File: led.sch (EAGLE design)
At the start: 46 parts, among them U1 TPS92513, U2 TPS92513

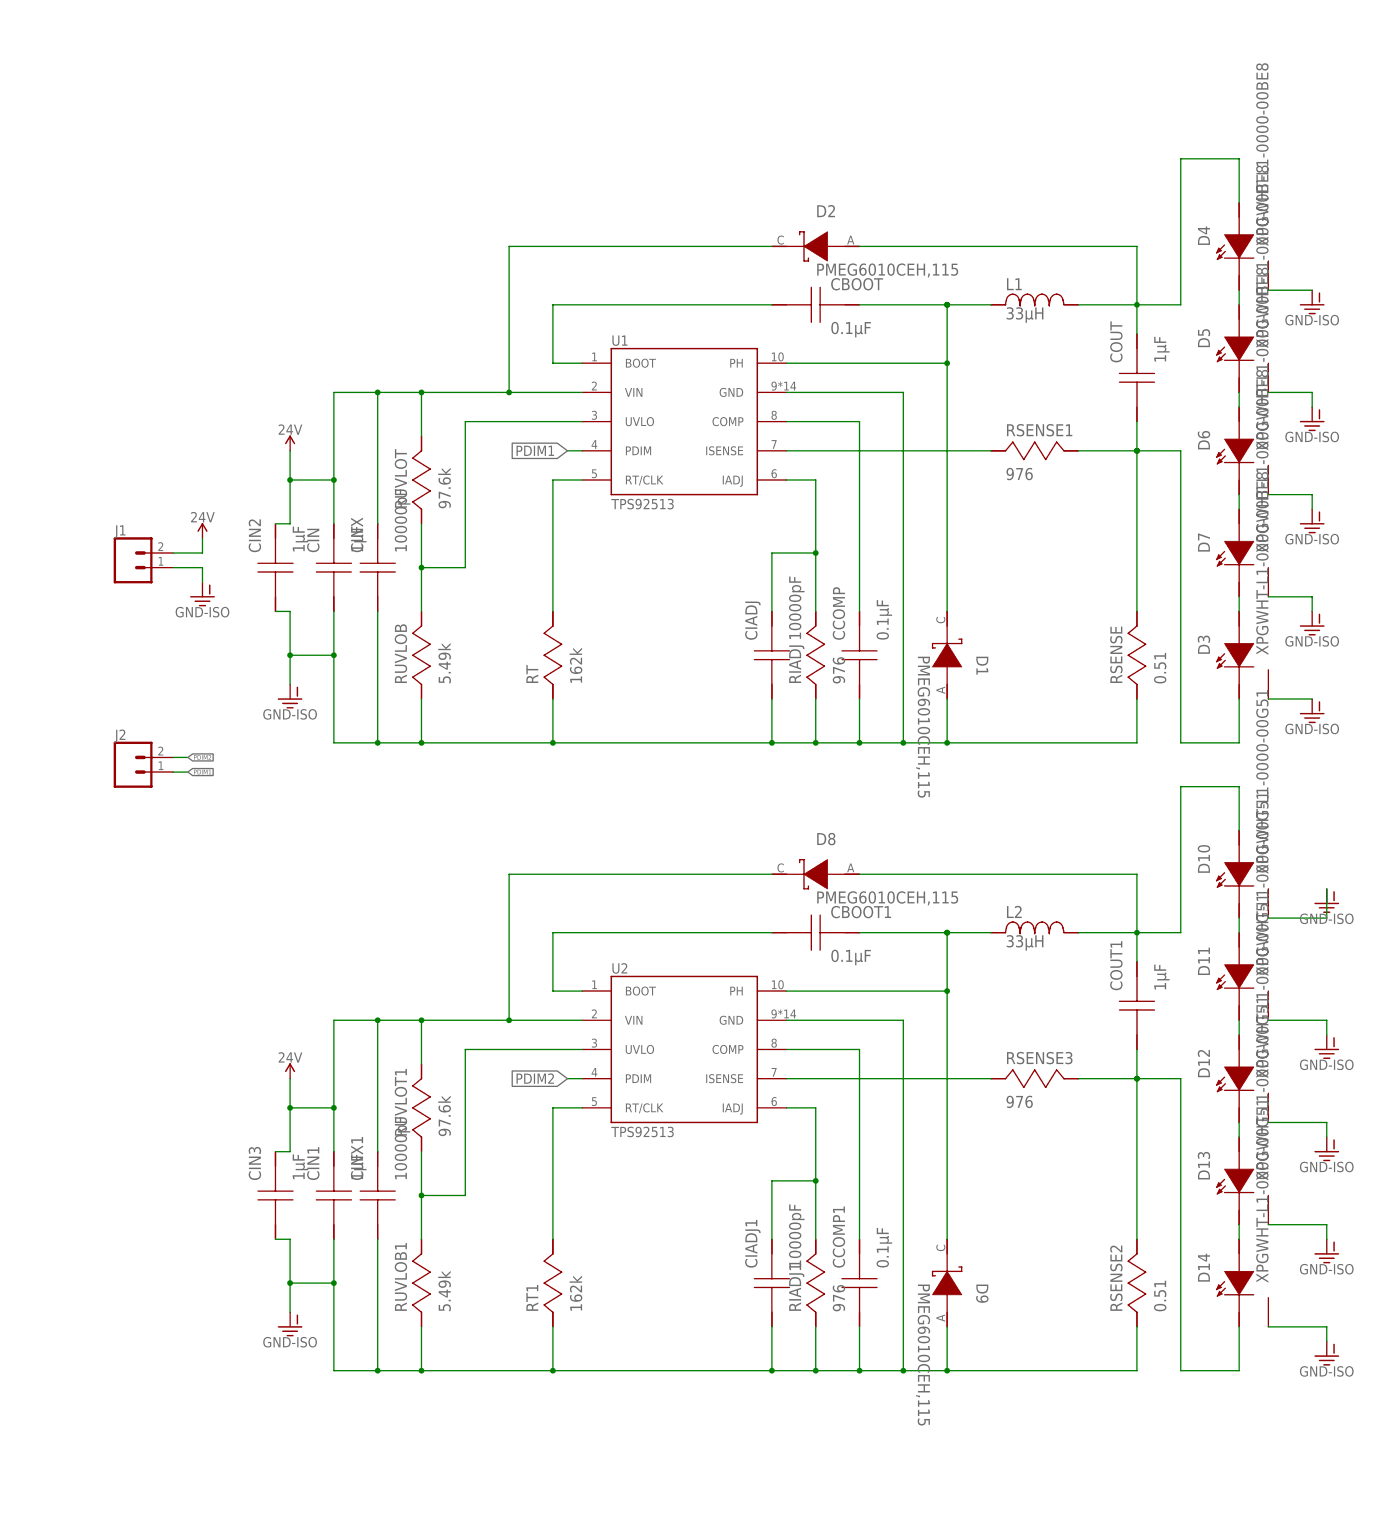
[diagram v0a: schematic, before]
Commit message: save
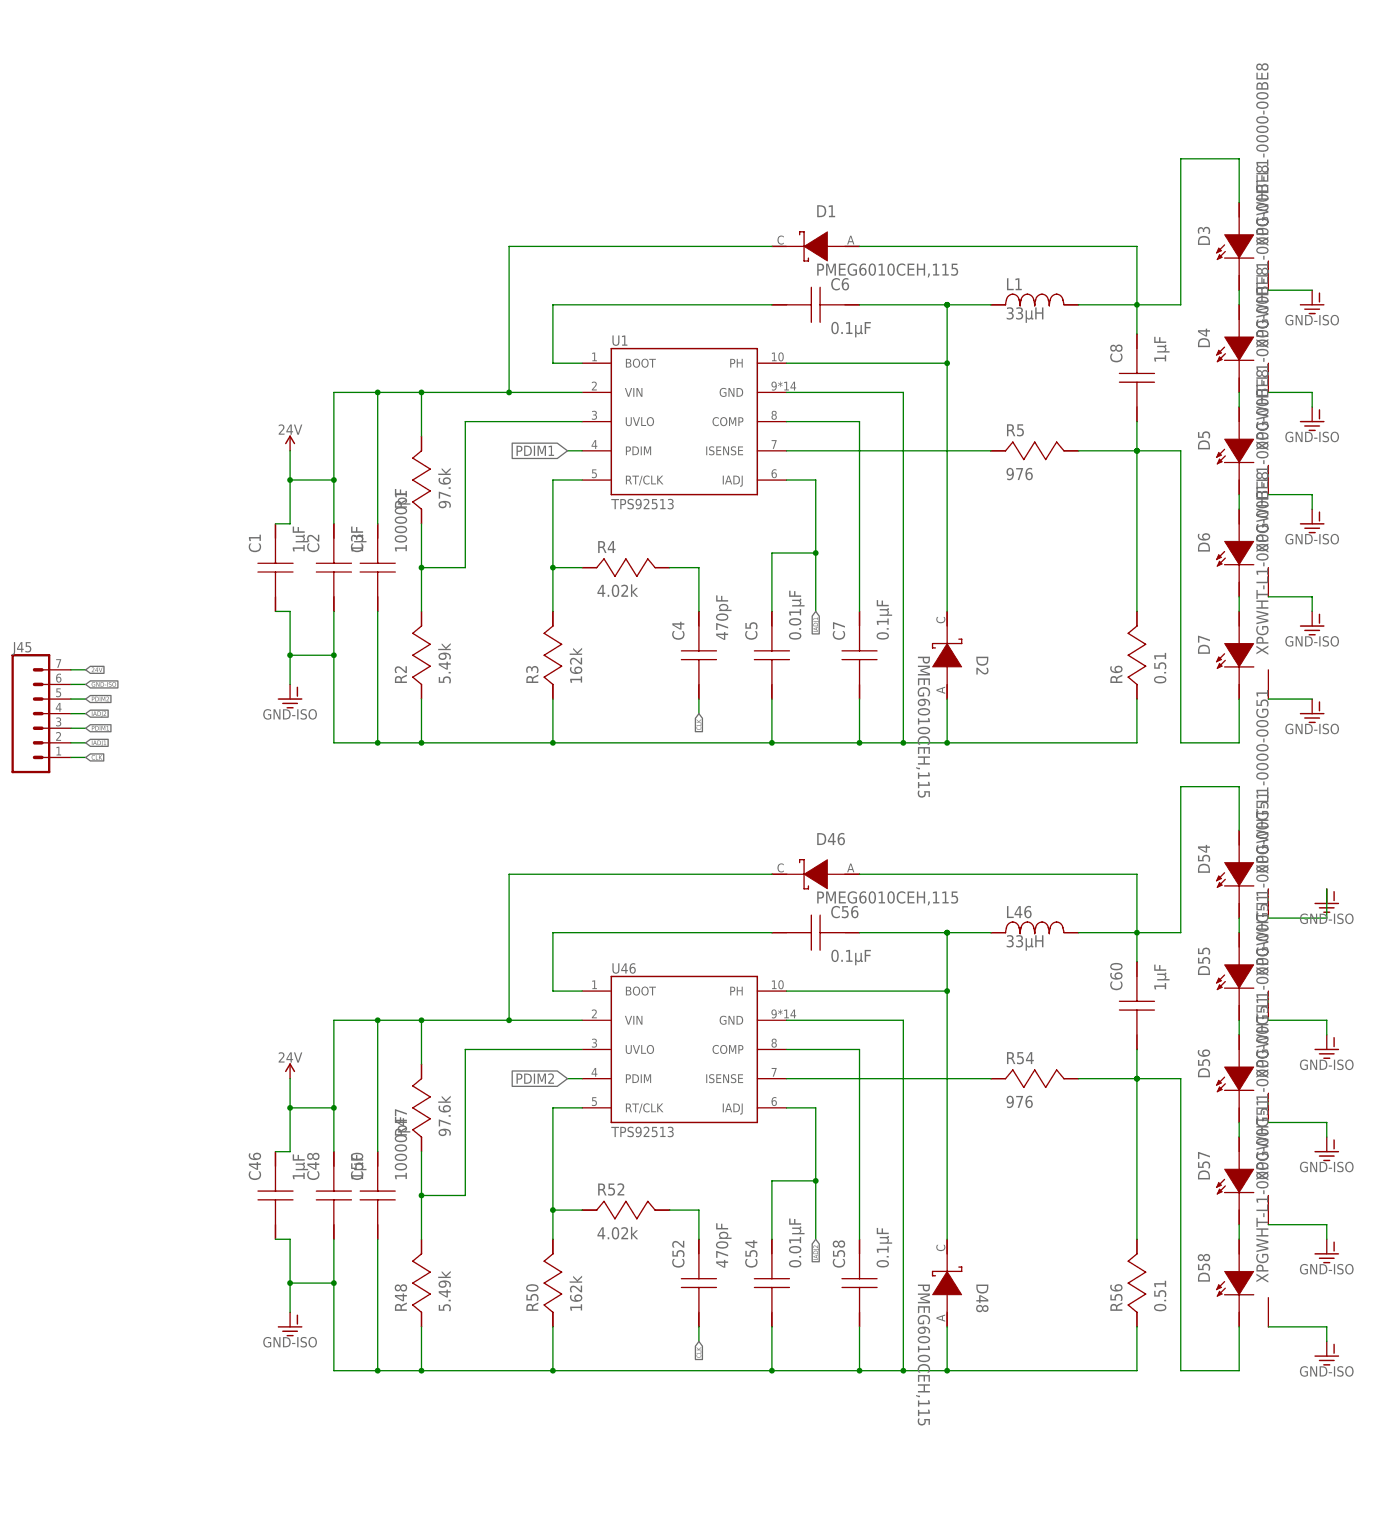
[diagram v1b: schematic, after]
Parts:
- removed CBOOT, CBOOT1: 0.1µF, derek:08053C104KAT2A
- removed J1, J2: (no value), derek:CONN_02
- removed RIADJ, RIADJ1: 976, derek:CRCW0402976RFKED
- added C4, C52: 470pF, derek:C0603X471K5RACTU
- added C56, C6: 0.1µF, derek:GRM188R71E104KA01D
- added J45: (no value), derek:CONN_07NO_SILK
- added R4, R52: 4.02k, derek:CRCW06034K02FKEA
- C5, C54: value 10000pF -> 0.01μF
- renumbered CCOMP to C7, CCOMP1 to C58, CIADJ to C5, CIADJ1 to C54, CIN to C2, CIN1 to C48, CIN2 to C1, CIN3 to C46, CINX to C3, CINX1 to C50, COUT to C8, COUT1 to C60, D10 to D54, D11 to D55, D12 to D56, D13 to D57, D14 to D58, D8 to D46, D9 to D48, L2 to L46, RSENSE to R6, RSENSE1 to R5, RSENSE2 to R56, RSENSE3 to R54, RT to R3, RT1 to R50, RUVLOB to R2, RUVLOB1 to R48, RUVLOT to R1, RUVLOT1 to R47, U2 to U46
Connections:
- removed net N$12 (its old number): D3.A, D7.C
- removed net N$2: C5.1, RIADJ.1, U1.IADJ
- removed net N$4: C54.1, RIADJ1.1, U46.IADJ
- new net CLK: C4.2, C52.2, J45.1
- new net IADJ1: C5.1, J45.2, U1.IADJ
- new net IADJ2: C54.1, J45.4, U46.IADJ
- new net N$13: D3.C, D4.A
- new net N$34: C4.1, R4.1
- new net N$36: C52.1, R52.1
- net 24V: now also D1.C, J45.7; no longer D2.C, J1.2
- net GND-ISO: now also D2.A, J45.6; no longer D1.A, J1.1, RIADJ.2, RIADJ1.2
- net N$10: now also C6.2; no longer CBOOT.2
- net N$16: now also C56.1; no longer CBOOT1.1
- net N$19: now also R52.2
- net N$21: now also C56.2; no longer CBOOT1.2
- net N$5: now also C6.1, D2.C; no longer CBOOT.1, D1.C
- net N$6: now also D7.C; no longer D3.C
- net N$7: now also D1.A, D3.A; no longer D2.A, D4.A
- net N$8: now also R4.2
- net PDIM1: now also J45.3; no longer J2.1
- net PDIM2: now also J45.5; no longer J2.2
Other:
- moved on the sheet: D1, D2, D3, D4, D5, D6, D7

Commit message: save
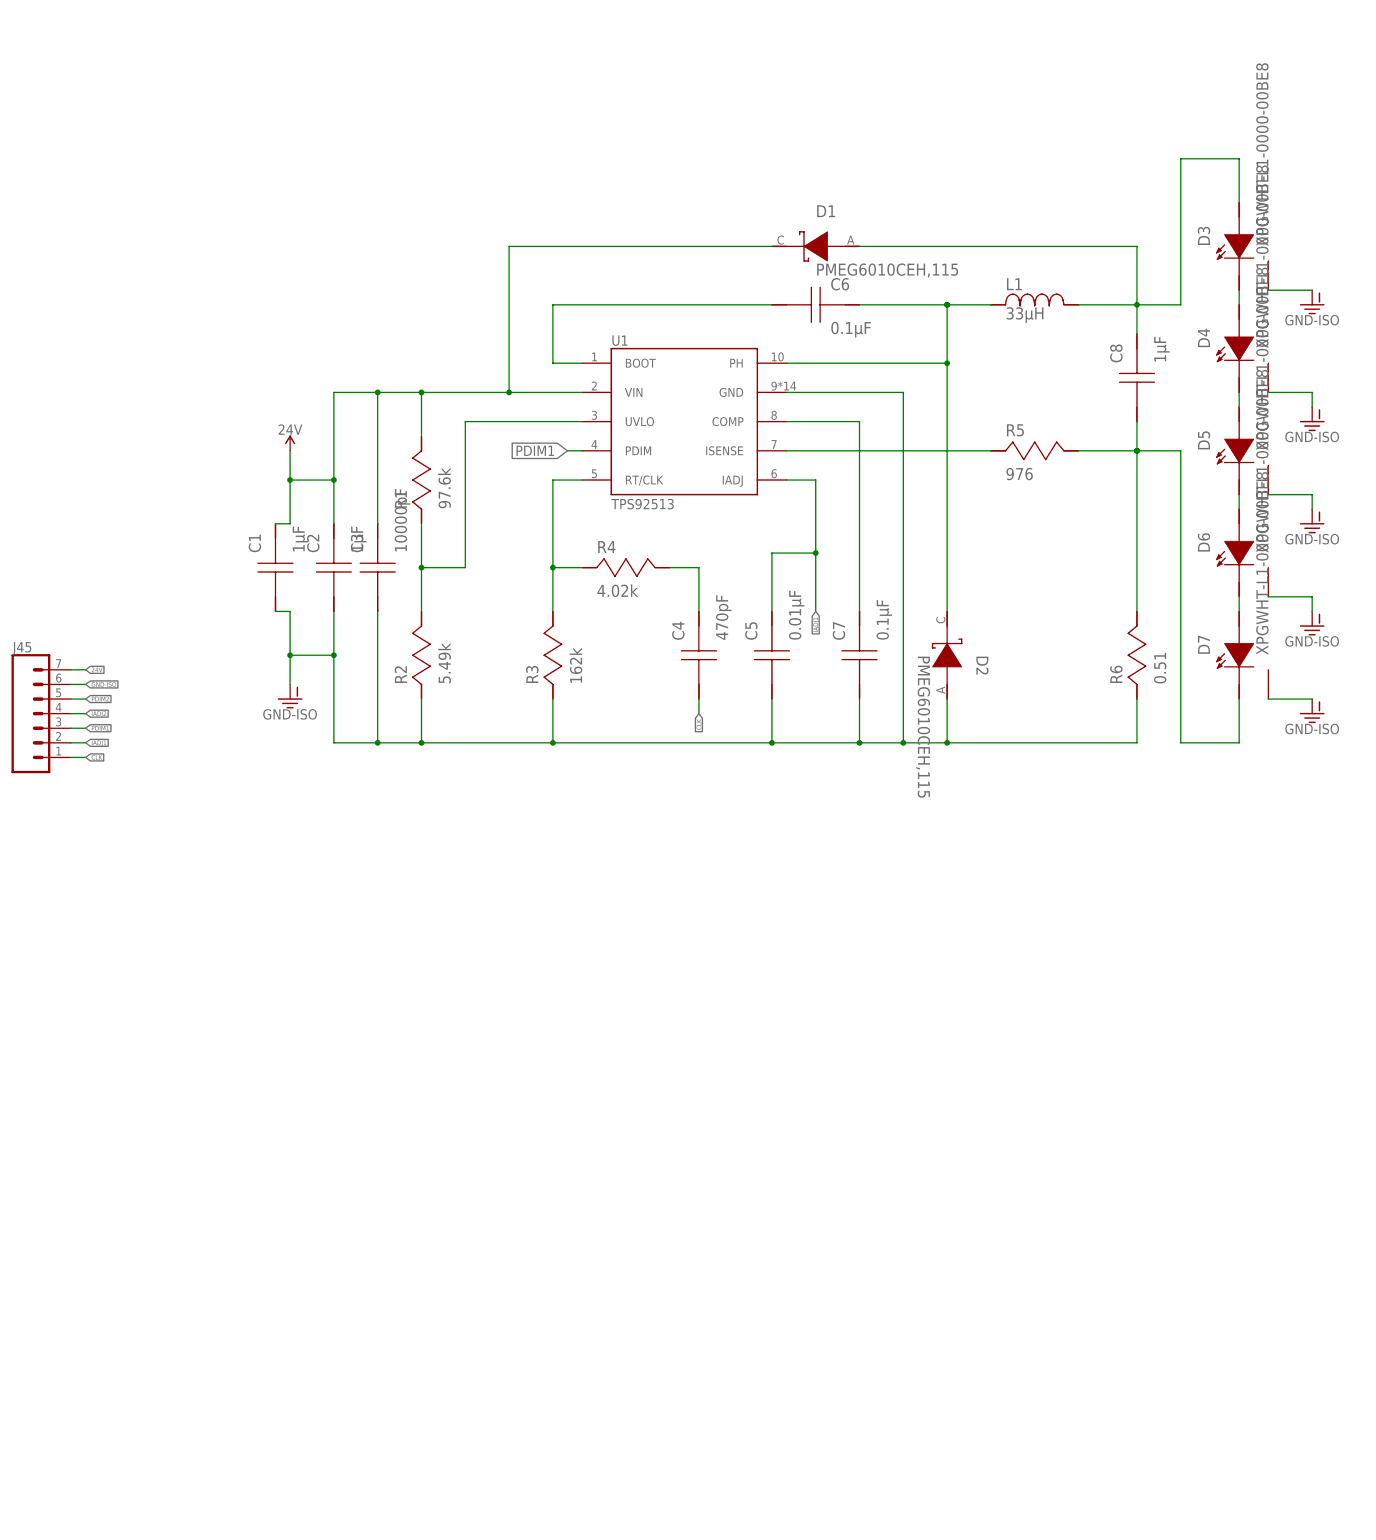
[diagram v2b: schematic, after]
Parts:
- removed C46, C48: 1µF, derek:GRM31MR71H105KA88L
- removed C50: 10000pF, derek:GCM155R71H103KA55D
- removed C52: 470pF, derek:C0603X471K5RACTU
- removed C54: 0.01μF, derek:CC0805KRX7R9BB103
- removed C56: 0.1µF, derek:GRM188R71E104KA01D
- removed C58: 0.1µF, derek:CC0805KRX7R8BB104
- removed C60: 1µF, derek:GMK212B7105KG-T
- removed D46, D48: PMEG6010CEH,115, derek:PMEG6010CEH,115
- removed D54, D55, D56, D57, D58: XPGWHT-L1-0000-00G51, derek:XPGWHT-L1-0000-00G51
- removed L46: 33µH, derek:SRN6045-330M
- removed R47: 97.6k, derek:CRCW040297K6FKED
- removed R48: 5.49k, derek:CRCW04025K49FKED
- removed R50: 162k, derek:CRCW0402162KFKED
- removed R52: 4.02k, derek:CRCW06034K02FKEA
- removed R54: 976, derek:CRCW0402976RFKED
- removed R56: 0.51, derek:CRM0805-FX-R510ELF
- removed U46: TPS92513, derek:TPS92513
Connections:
- removed net N$1: R47.2, R48.1, U46.UVLO
- removed net N$16: C56.1, D48.C, L46.1, U46.PH
- removed net N$17: C60.2, D58.C, R54.1, R56.1
- removed net N$18: C60.1, D46.A, D54.A, L46.2
- removed net N$19: R50.1, R52.2, U46.RT/CLK
- removed net N$20: C58.1, U46.COMP
- removed net N$21: C56.2, U46.BOOT
- removed net N$22: R54.2, U46.ISENSE
- removed net N$23: D54.C, D55.A
- removed net N$24: D55.C, D56.A
- removed net N$25: D56.C, D57.A
- removed net N$26: D57.C, D58.A
- removed net N$36: C52.1, R52.1
- net 24V: no longer C46.1, C48.1, C50.1, D46.C, R47.1, U46.VIN
- net CLK: no longer C52.2
- net GND-ISO: no longer C46.2, C48.2, C50.2, C54.2, C58.2, D48.A, D54.GND, D55.GND, D56.GND, D57.GND, D58.GND, R48.2, R50.2, R56.2, U46.GND
- net IADJ2: no longer C54.1, U46.IADJ
- net PDIM2: no longer U46.PDIM

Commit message: save
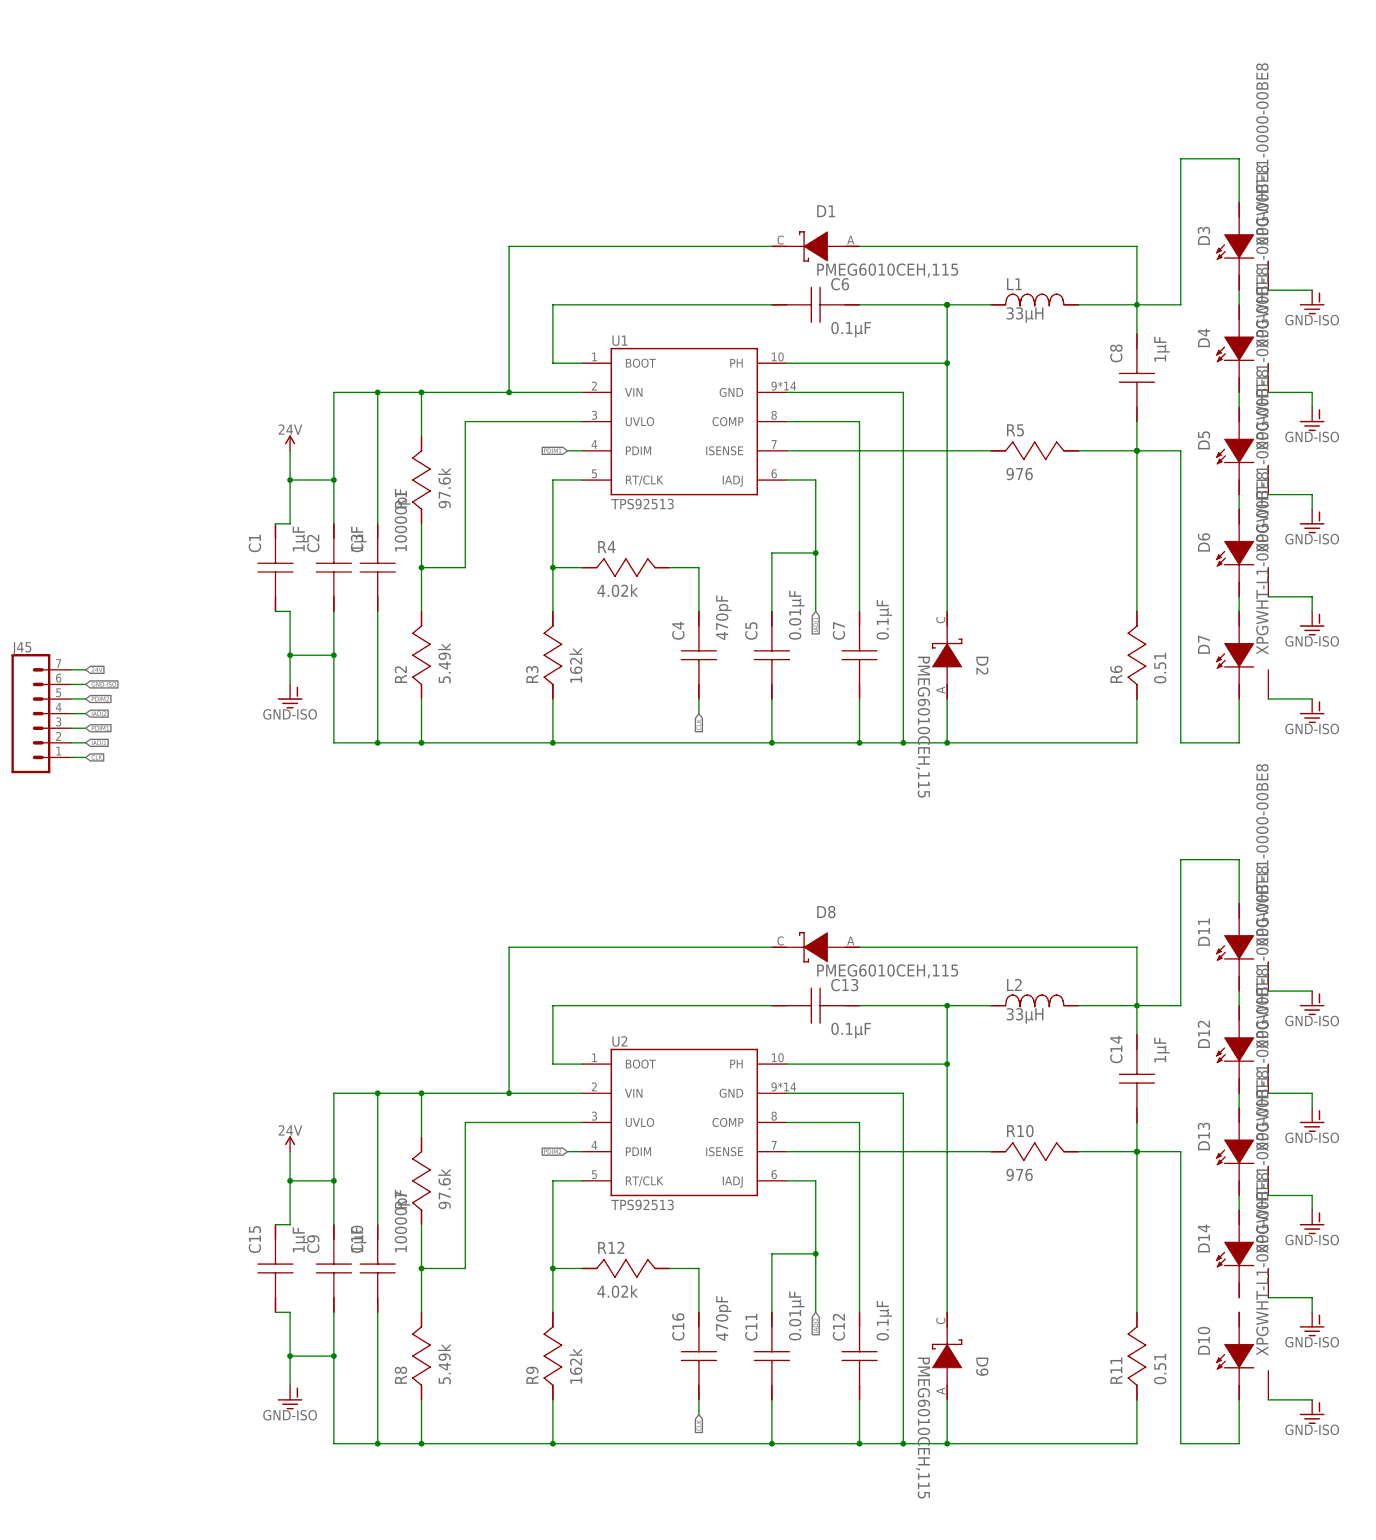
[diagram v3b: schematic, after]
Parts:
- added C10: 10000pF, derek:GCM155R71H103KA55D
- added C11: 0.01μF, derek:CC0805KRX7R9BB103
- added C12: 0.1µF, derek:CC0805KRX7R8BB104
- added C13: 0.1µF, derek:GRM188R71E104KA01D
- added C14: 1µF, derek:GMK212B7105KG-T
- added C15, C9: 1µF, derek:GRM31MR71H105KA88L
- added C16: 470pF, derek:C0603X471K5RACTU
- added D10, D11, D12, D13, D14: XPGWHT-L1-0000-00BE8, derek:XPGWHT-L1-0000-00BE8
- added D8, D9: PMEG6010CEH,115, derek:PMEG6010CEH,115
- added L2: 33µH, derek:SRN6045-330M
- added R10: 976, derek:CRCW0402976RFKED
- added R11: 0.51, derek:CRM0805-FX-R510ELF
- added R12: 4.02k, derek:CRCW06034K02FKEA
- added R7: 97.6k, derek:CRCW040297K6FKED
- added R8: 5.49k, derek:CRCW04025K49FKED
- added R9: 162k, derek:CRCW0402162KFKED
- added U2: TPS92513, derek:TPS92513
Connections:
- new net N$1: R7.2, R8.1, U2.UVLO
- new net N$16: C13.1, D9.C, L2.1, U2.PH
- new net N$17: R12.2, R9.1, U2.RT/CLK
- new net N$18: C12.1, U2.COMP
- new net N$19: C13.2, U2.BOOT
- new net N$2: D11.C, D12.A
- new net N$20: R10.2, U2.ISENSE
- new net N$21: D12.C, D13.A
- new net N$22: D13.C, D14.A
- new net N$23: C14.1, D11.A, D8.A, L2.2
- new net N$25: C16.1, R12.1
- new net N$4: C14.2, D10.C, R10.1, R11.1
- net 24V: now also C10.1, C15.1, C9.1, D8.C, R7.1, U2.VIN
- net CLK: now also C16.2
- net GND-ISO: now also C10.2, C11.2, C12.2, C15.2, C9.2, D10.GND, D11.GND, D12.GND, D13.GND, D14.GND, D9.A, R11.2, R8.2, R9.2, U2.GND
- net IADJ2: now also C11.1, U2.IADJ
- net PDIM2: now also U2.PDIM
